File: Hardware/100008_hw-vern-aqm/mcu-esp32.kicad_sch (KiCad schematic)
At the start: 14 parts

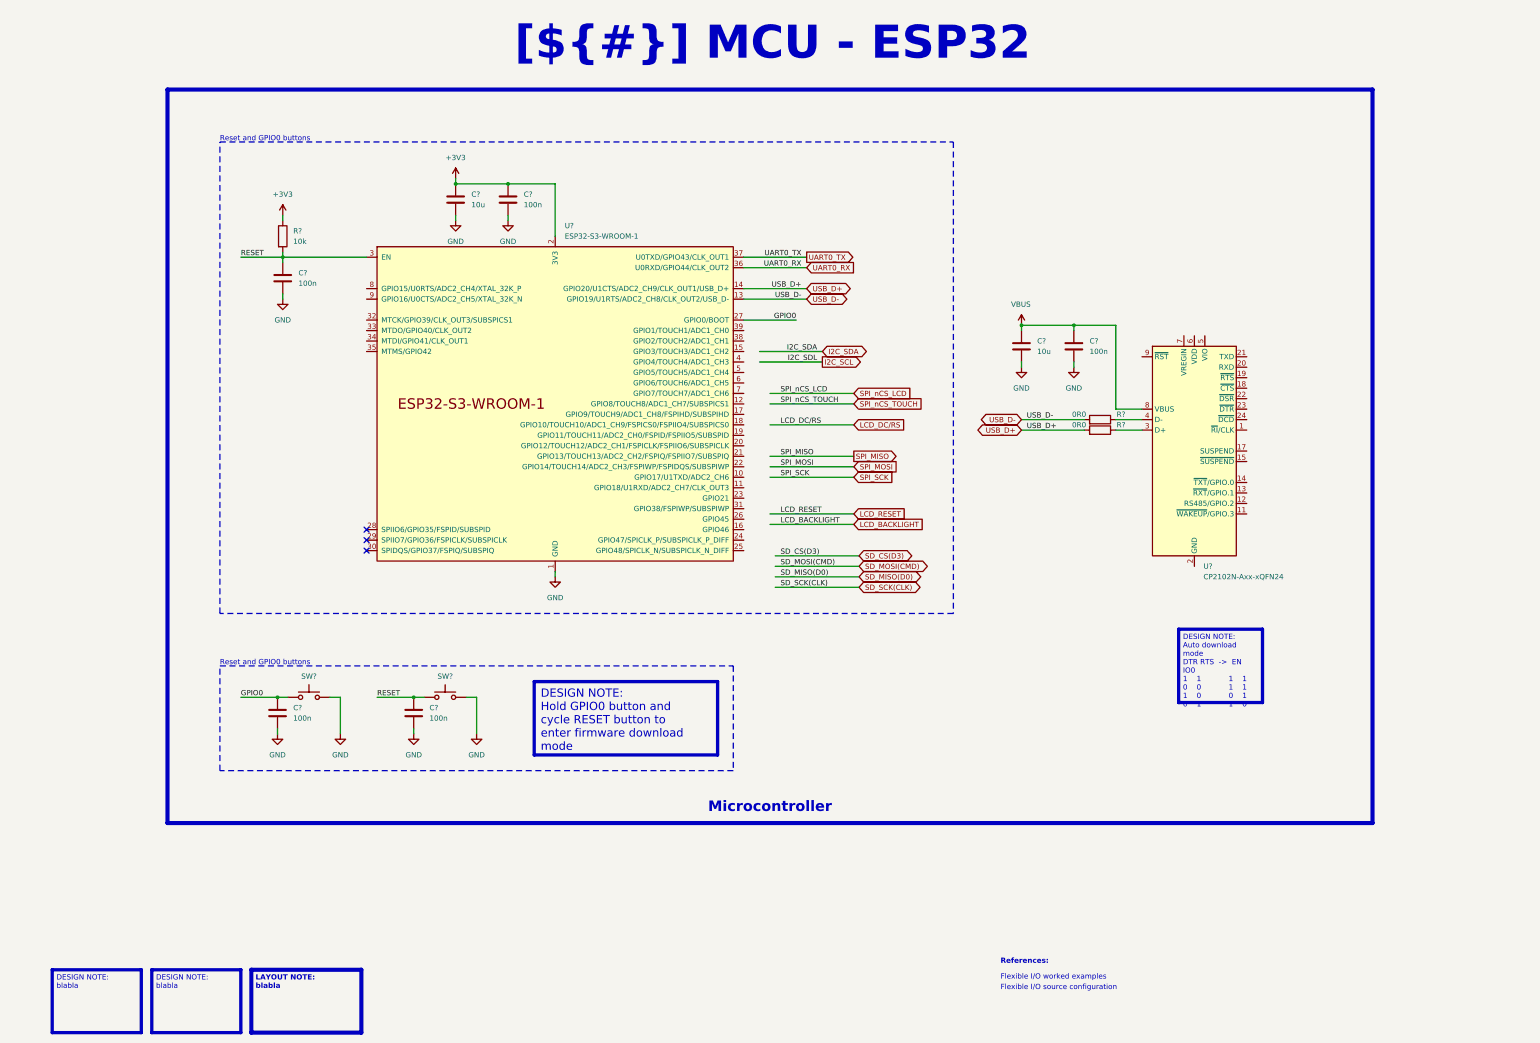
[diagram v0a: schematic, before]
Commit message: schematic and pcb layout
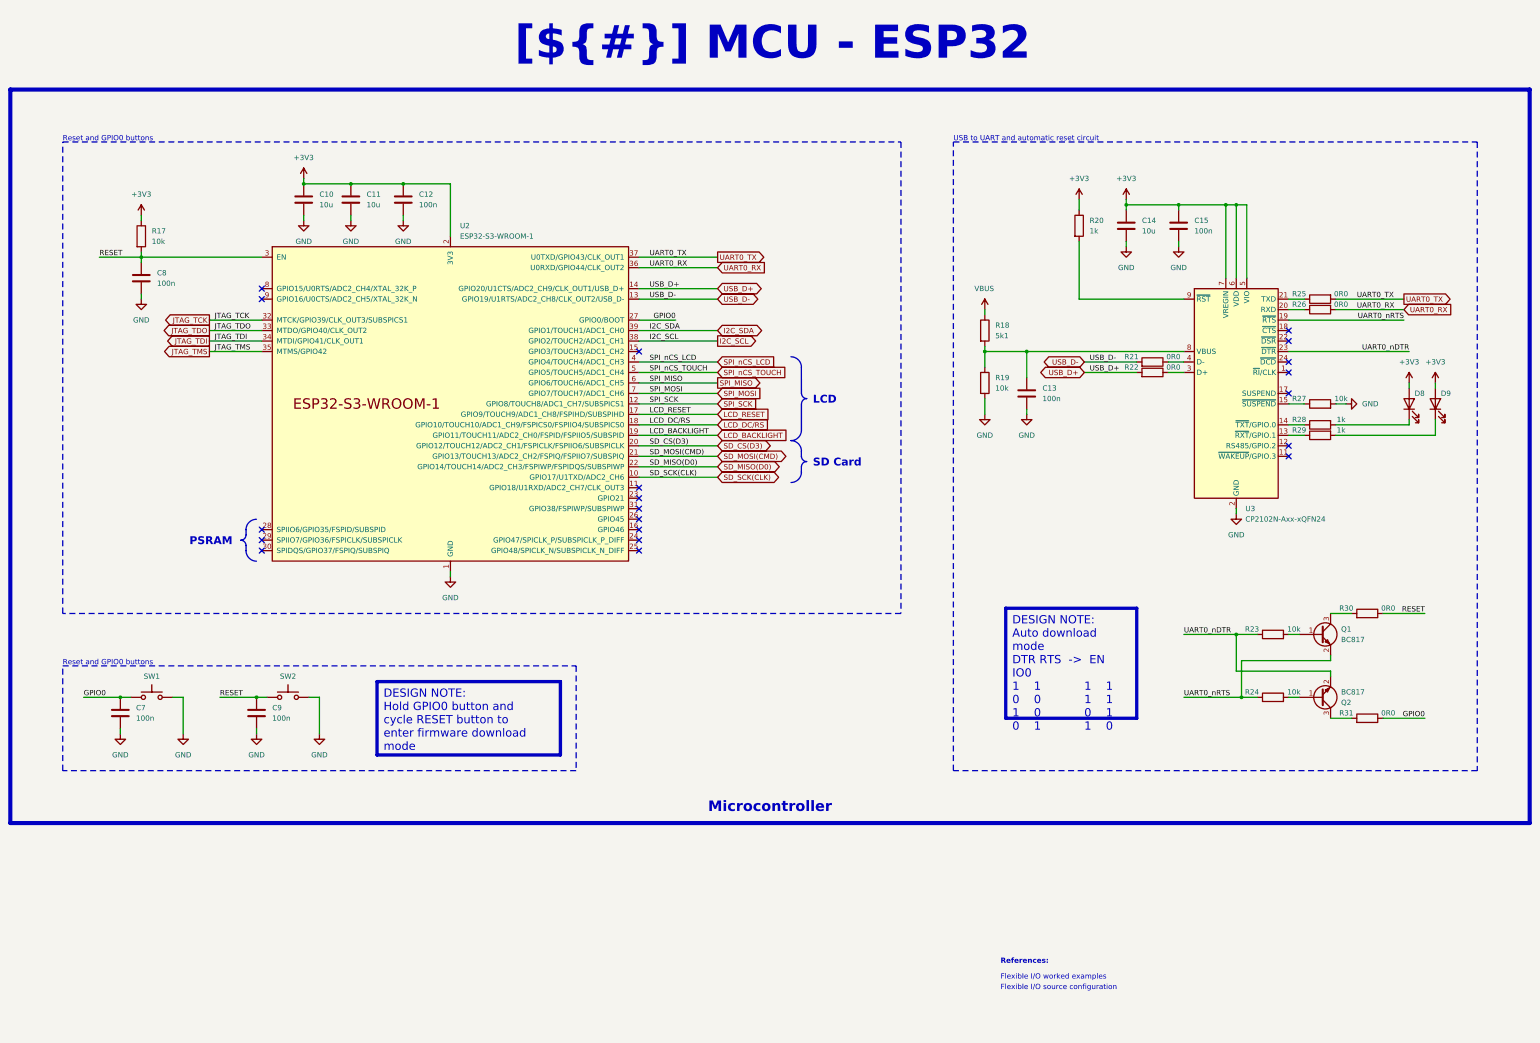
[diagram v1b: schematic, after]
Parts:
- added C10: 10u, Capacitor_SMD:C_0805_2012Metric, symbol Device:C
- added C13: 100n, Capacitor_SMD:C_0603_1608Metric, symbol Device:C
- added D8, D9: LED, LED_SMD:LED_0603_1608Metric, symbol Device:LED
- added Q1, Q2: BC817, Package_TO_SOT_SMD:SOT-23, symbol Transistor_BJT:BC817
- added R18: 5k1, Resistor_SMD:R_0603_1608Metric, symbol Device:R
- added R19, R23, R24, R27: 10k, Resistor_SMD:R_0603_1608Metric, symbol Device:R
- added R20, R28, R29: 1k, Resistor_SMD:R_0603_1608Metric, symbol Device:R
- added R25, R26, R30, R31: 0R0, Resistor_SMD:R_0603_1608Metric, symbol Device:R
- gave numbers to parts that had none: 14
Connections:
- net +3V3: now also C14.1, C15.1, U3.5 (VIO), U3.6 (VDD), U3.7 (VREGIN), C10.1, D8.2 (A), D9.2 (A), R20.1
- net GND: now also U3.2 (GND), U3.25 (GND), C10.2, C13.2, R19.2, R27.2
- net GPIO0: now also R31.1
- net I2C_SCL: now also U2.38 (GPIO2/TOUCH2/ADC1_CH1)
- net I2C_SDA: now also U2.39 (GPIO1/TOUCH1/ADC1_CH0)
- net LCD_BACKLIGHT: now also U2.19 (GPIO11/TOUCH11/ADC2_CH0/FSPID/FSPIIO5/SUBSPID)
- net LCD_DC/RS: now also U2.18 (GPIO10/TOUCH10/ADC1_CH9/FSPICS0/FSPIIO4/SUBSPICS0)
- net LCD_RESET: now also U2.17 (GPIO9/TOUCH9/ADC1_CH8/FSPIHD/SUBSPIHD)
- net RESET: now also R30.1
- net SD_CS(D3): now also U2.20 (GPIO12/TOUCH12/ADC2_CH1/FSPICLK/FSPIIO6/SUBSPICLK)
- net SD_MISO(D0): now also U2.22 (GPIO14/TOUCH14/ADC2_CH3/FSPIWP/FSPIDQS/SUBSPIWP)
- net SD_MOSI(CMD): now also U2.21 (GPIO13/TOUCH13/ADC2_CH2/FSPIQ/FSPIIO7/SUBSPIQ)
- net SD_SCK(CLK): now also U2.10 (GPIO17/U1TXD/ADC2_CH6)
- net SPI_MISO: now also U2.6 (GPIO6/TOUCH6/ADC1_CH5)
- net SPI_MOSI: now also U2.7 (GPIO7/TOUCH7/ADC1_CH6)
- net SPI_SCK: now also U2.12 (GPIO8/TOUCH8/ADC1_CH7/SUBSPICS1)
- net SPI_nCS_LCD: now also U2.4 (GPIO4/TOUCH4/ADC1_CH3)
- net SPI_nCS_TOUCH: now also U2.5 (GPIO5/TOUCH5/ADC1_CH4)
- net UART0_RX: now also R26.2
- net UART0_TX: now also R25.2
- net VBUS: now also R18.1; no longer C14.1, C15.1, U3.8 (VBUS)
- net at U3.13 (~{RXT}/GPIO.1): now also R29.1
- net at U3.14 (~{TXT}/GPIO.0): now also R28.1
- net at U3.15 (~{SUSPEND}): now also R27.1
- net UART0_nRTS: now reaches U3.19 (~{RTS})
- net UART0_nRTS: now also Q1.2 (E), R24.1
- net at U3.20 (RXD): now also R26.1
- net at U3.21 (TXD): now also R25.1
- net UART0_nDTR: now reaches U3.23 (~{DTR})
- net UART0_nDTR: now also Q2.2 (E), R23.1
- net at U3.9 (~{RST}): now also R20.2
- net JTAG_TCK: now reaches U2.32 (MTCK/GPIO39/CLK_OUT3/SUBSPICS1)
- net JTAG_TDO: now reaches U2.33 (MTDO/GPIO40/CLK_OUT2)
- net JTAG_TDI: now reaches U2.34 (MTDI/GPIO41/CLK_OUT1)
- net JTAG_TMS: now reaches U2.35 (MTMS/GPIO42)
- new net: C13.1, R18.2, R19.1, U3.8 (VBUS)
- new net: D9.1 (K), R29.2
- new net: Q1.1 (B), R23.2
- new net: Q1.3 (C), R30.2
- new net: Q2.1 (B), R24.2
- new net: Q2.3 (C), R31.2
- new net: D8.1 (K), R28.2
- no-connect marks 3 -> 20
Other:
- note added: "USB to UART and automatic reset circuit"
- moved on the sheet: C11, C12, C14, C15, C7, C8, C9, R17, R21, R22, SW1, SW2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

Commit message: schematic, pcb layout, added mouser shoping cart
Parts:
- Q1, Q2: footprint Package_TO_SOT_SMD:SOT-23 -> Package_TO_SOT_SMD:SOT-323_SC-70
